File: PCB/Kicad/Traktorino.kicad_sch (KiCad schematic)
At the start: 5 parts, among them J1 analog_pins, J2 mux_pins, J3 595_pins, J4 d13

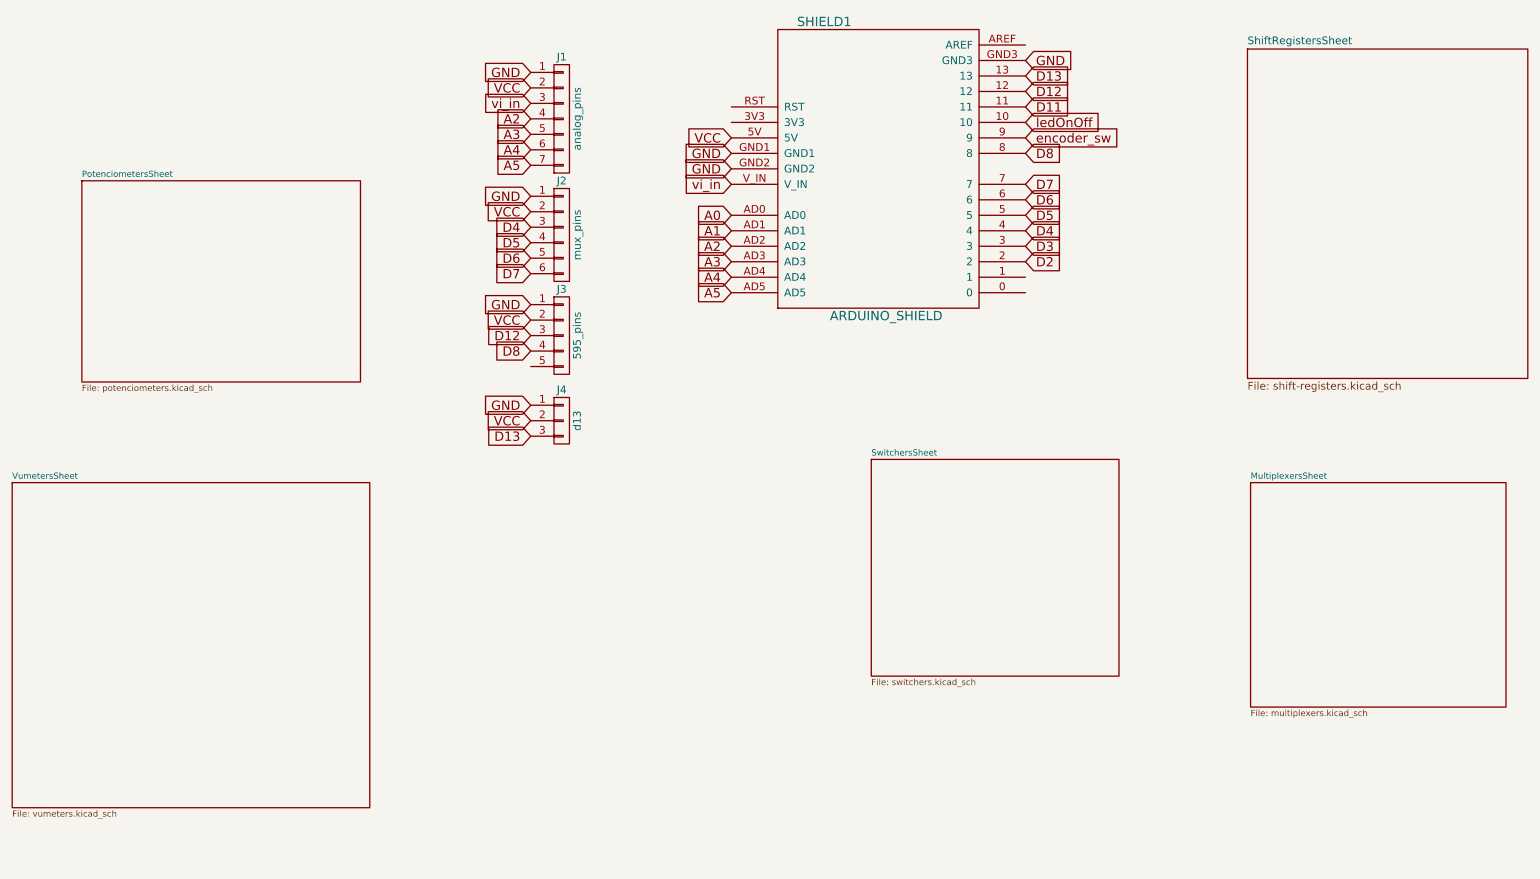
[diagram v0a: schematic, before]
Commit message: update elements WIP
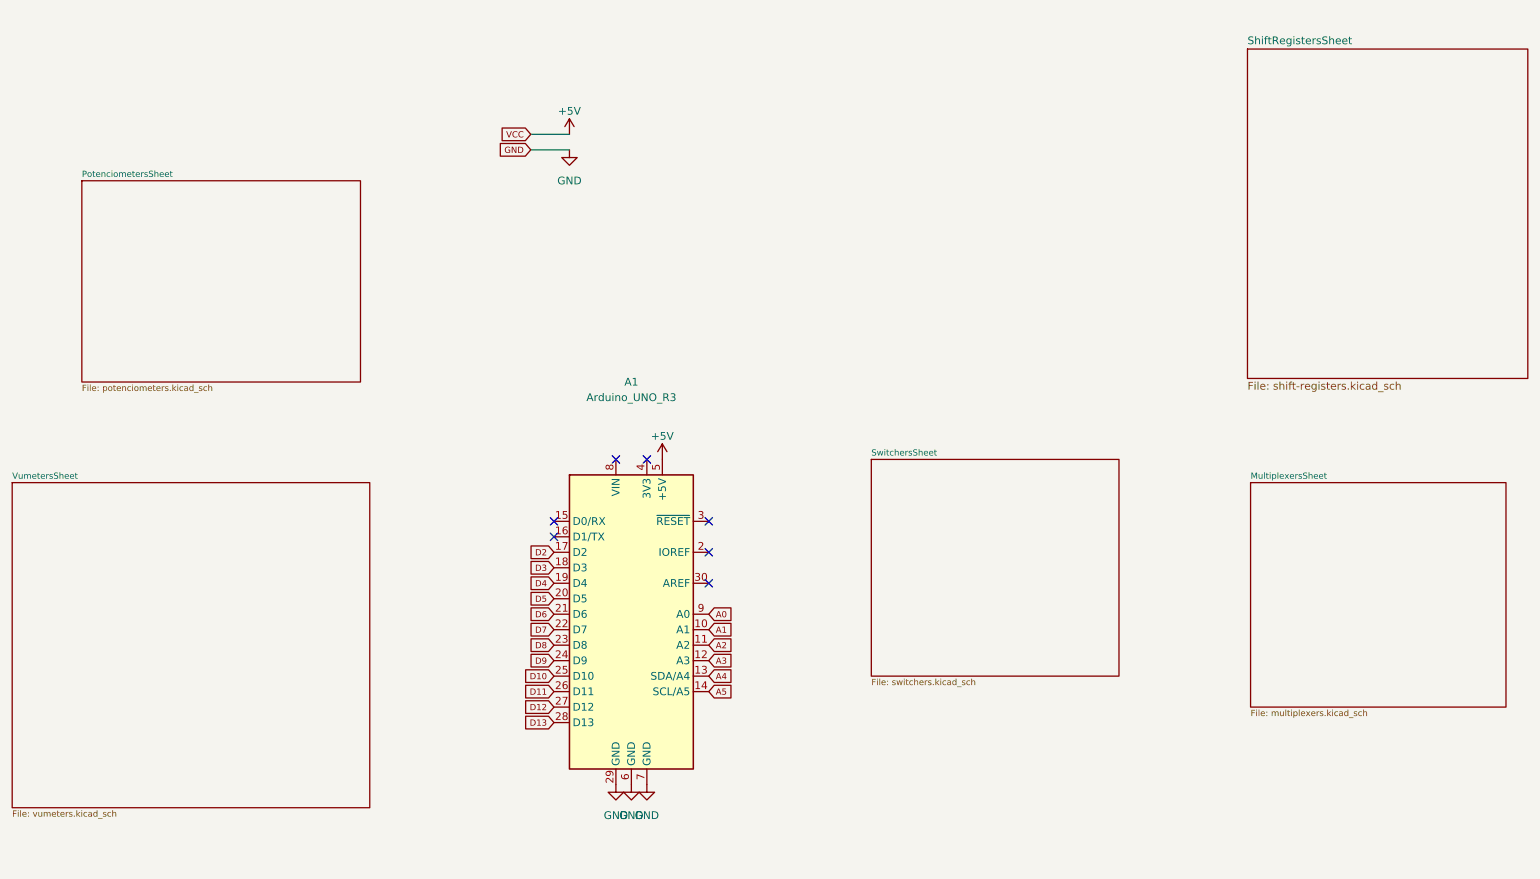
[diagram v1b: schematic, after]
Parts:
- removed J1: analog_pins, Pin_Headers:Pin_Header_Straight_1x07_Pitch2.54mm, symbol Traktorino-rescue:CONN_01X07
- removed J2: mux_pins, Pin_Headers:Pin_Header_Straight_1x06_Pitch2.54mm, symbol Traktorino-rescue:CONN_01X06
- removed J3: 595_pins, Pin_Headers:Pin_Header_Straight_1x05_Pitch2.54mm, symbol Traktorino-rescue:CONN_01X05
- removed J4: d13, Pin_Headers:Pin_Header_Straight_1x03_Pitch2.54mm, symbol Traktorino-rescue:CONN_01X03
- removed SHIELD1: ARDUINO_SHIELD, arduino_shields:ARDUINO_SHIELD_2_040pins, symbol Traktorino-rescue:ARDUINO_SHIELD
- added A1: Arduino_UNO_R3, Module:Arduino_UNO_R2, symbol MCU_Module:Arduino_UNO_R2
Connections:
- net A0: now also A1.9 (A0)
- net A1: now also A1.10 (A1)
- net A2: now also A1.11 (A2)
- net A3: now also A1.12 (A3)
- net A4: now also A1.13 (SDA/A4)
- net A5: now also A1.14 (SCL/A5)
- net D11: now also A1.26 (D11)
- net D12: now also A1.27 (D12)
- net D13: now also A1.28 (D13)
- net D2: now also A1.17 (D2)
- net D3: now also A1.18 (D3)
- net D4: now also A1.19 (D4)
- net D5: now also A1.20 (D5)
- net D6: now also A1.21 (D6)
- net D7: now also A1.22 (D7)
- net D8: now also A1.23 (D8)
- net GND: now also A1.29 (GND), A1.6 (GND), A1.7 (GND)
- new net +5V: A1.5 (+5V)
- new net D10: A1.25 (D10)
- new net D9: A1.24 (D9)
- no-connect marks 0 -> 7

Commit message: progress
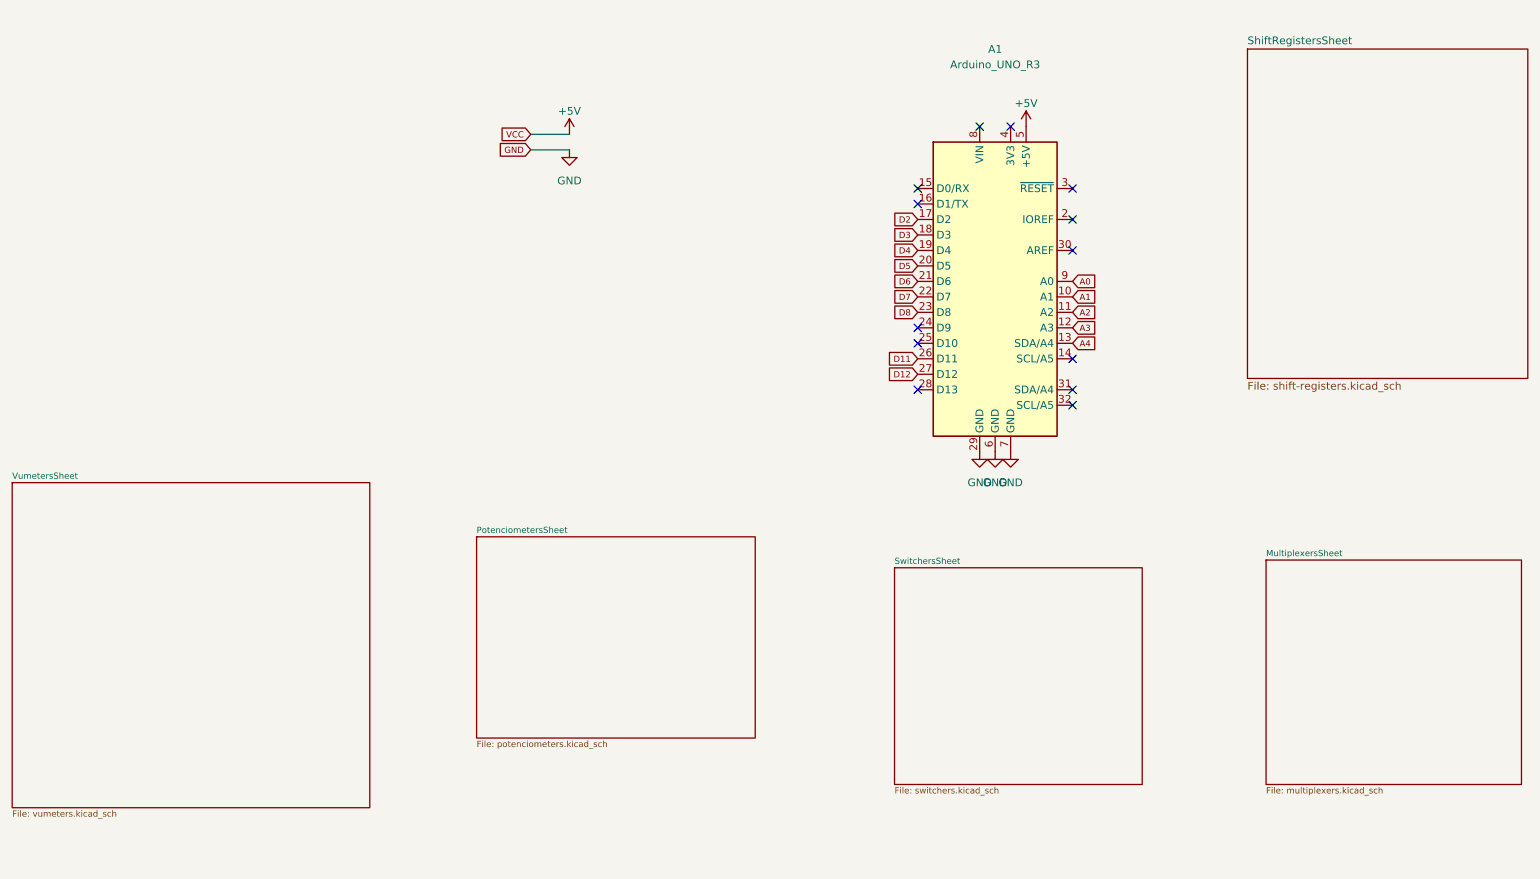
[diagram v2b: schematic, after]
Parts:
- A1: footprint Module:Arduino_UNO_R2 -> Module:Arduino_UNO_R3_WithMountingHoles; symbol MCU_Module:Arduino_UNO_R2 -> MCU_Module:Arduino_UNO_R3
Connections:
- net A5: no longer names the net of A1.14 (SCL/A5)
- net D10: no longer names the net of A1.25 (D10)
- net D13: no longer names the net of A1.28 (D13)
- net D9: no longer names the net of A1.24 (D9)
- no-connect marks 7 -> 13

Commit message: mod layout
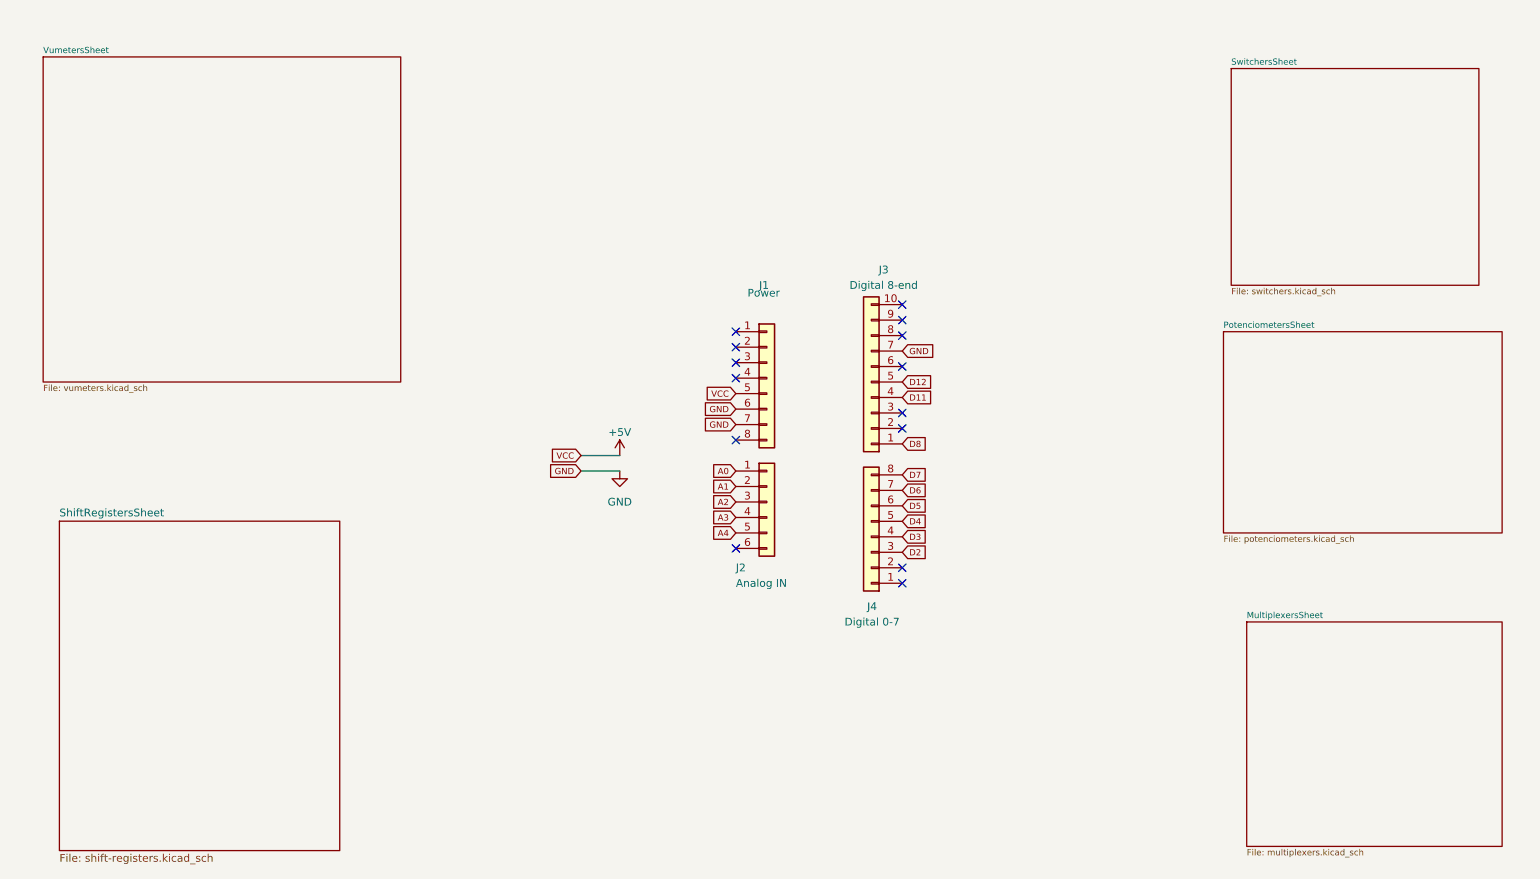
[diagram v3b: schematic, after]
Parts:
- removed A1: Arduino_UNO_R3, Module:Arduino_UNO_R3_WithMountingHoles, symbol MCU_Module:Arduino_UNO_R3
- added J1: Power, Connector_PinHeader_2.54mm:PinHeader_1x08_P2.54mm_Vertical, symbol Connector_Generic:Conn_01x08
- added J2: Analog IN, Connector_PinHeader_2.54mm:PinHeader_1x06_P2.54mm_Vertical, symbol Connector_Generic:Conn_01x06
- added J3: Digital 8-end, Connector_PinHeader_2.54mm:PinHeader_1x10_P2.54mm_Vertical, symbol Connector_Generic:Conn_01x10
- added J4: Digital 0-7, Connector_PinHeader_2.54mm:PinHeader_1x08_P2.54mm_Vertical, symbol Connector_Generic:Conn_01x08
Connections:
- net +5V: now also J1.5 (Pin_5)
- net A0: now also J2.1 (Pin_1)
- net A1: now also J2.2 (Pin_2)
- net A2: now also J2.3 (Pin_3)
- net A3: now also J2.4 (Pin_4)
- net A4: now also J2.5 (Pin_5)
- net D11: now also J3.4 (Pin_4)
- net D12: now also J3.5 (Pin_5)
- net D2: now also J4.3 (Pin_3)
- net D3: now also J4.4 (Pin_4)
- net D4: now also J4.5 (Pin_5)
- net D5: now also J4.6 (Pin_6)
- net D6: now also J4.7 (Pin_7)
- net D7: now also J4.8 (Pin_8)
- net D8: now also J3.1 (Pin_1)
- net GND: now also J1.6 (Pin_6), J1.7 (Pin_7), J3.7 (Pin_7)
- no-connect marks 13 -> 14
